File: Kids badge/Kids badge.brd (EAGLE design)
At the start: 3 parts

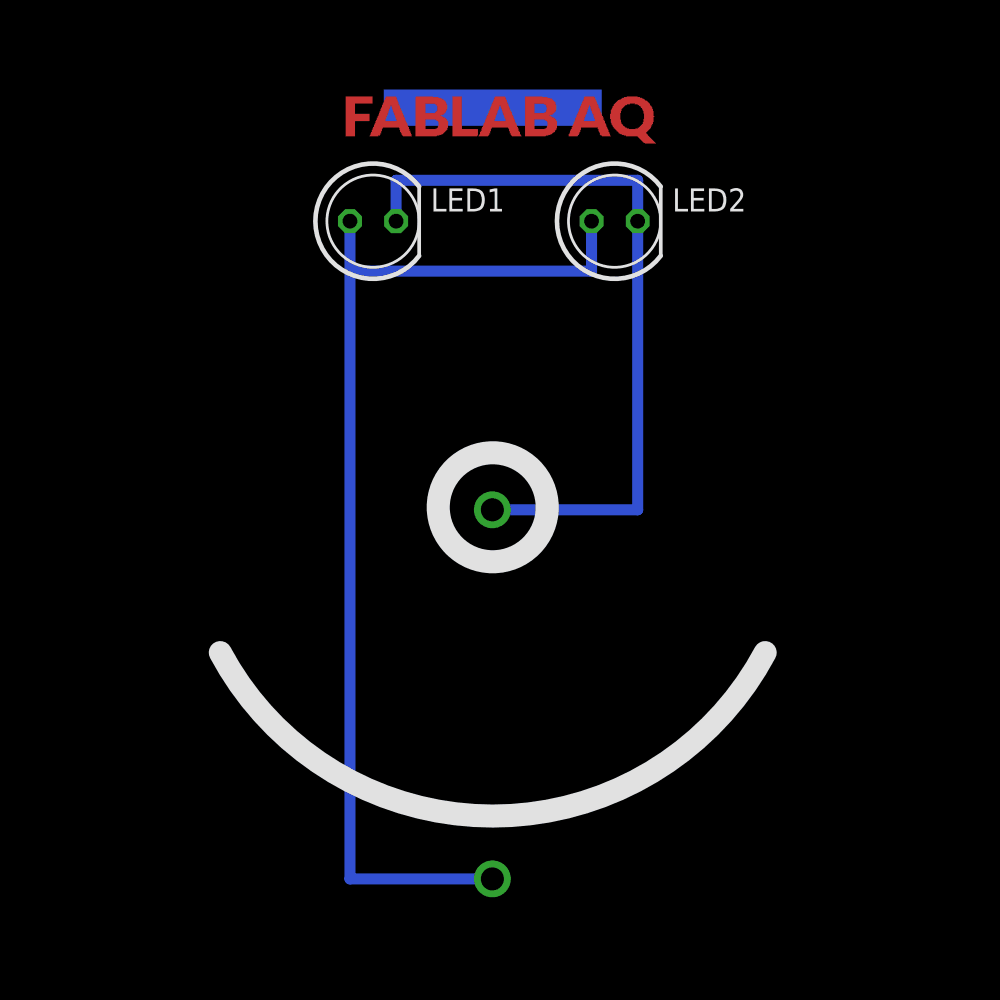
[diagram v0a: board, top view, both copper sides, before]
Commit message: new badges
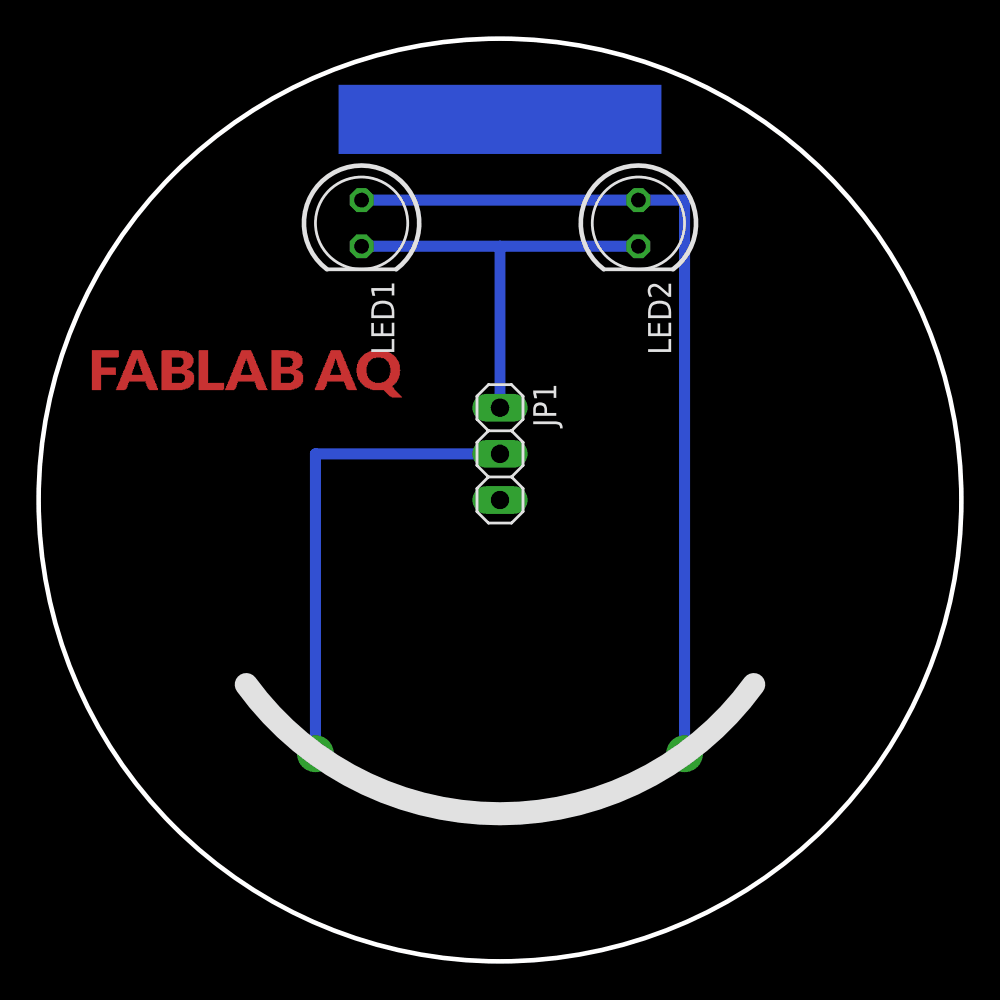
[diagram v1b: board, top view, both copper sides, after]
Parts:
- added JP1: (no value), pinhead:1X03
- BATT: value (none) -> BATTERY_1236_C
- moved BATT 12.6 mm to (35.6, 11.4), turned to 270 degrees
- moved LED2 1.31 mm to (33.0, 40.6), turned to 270 degrees
- moved LED1 0.64 mm to (17.8, 40.6), turned to 270 degrees
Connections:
- new net N$3: BATT.-, JP1.2
- net N$2: now also JP1.1; no longer BATT.-
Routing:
- net N$3: track 0.00 -> 26.7 mm
- net N$2: track 41.7 -> 24.1 mm
- net N$1: track 60.1 -> 48.3 mm
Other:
- board outline added: 50.8 x 50.8 mm

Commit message: routed PCBs
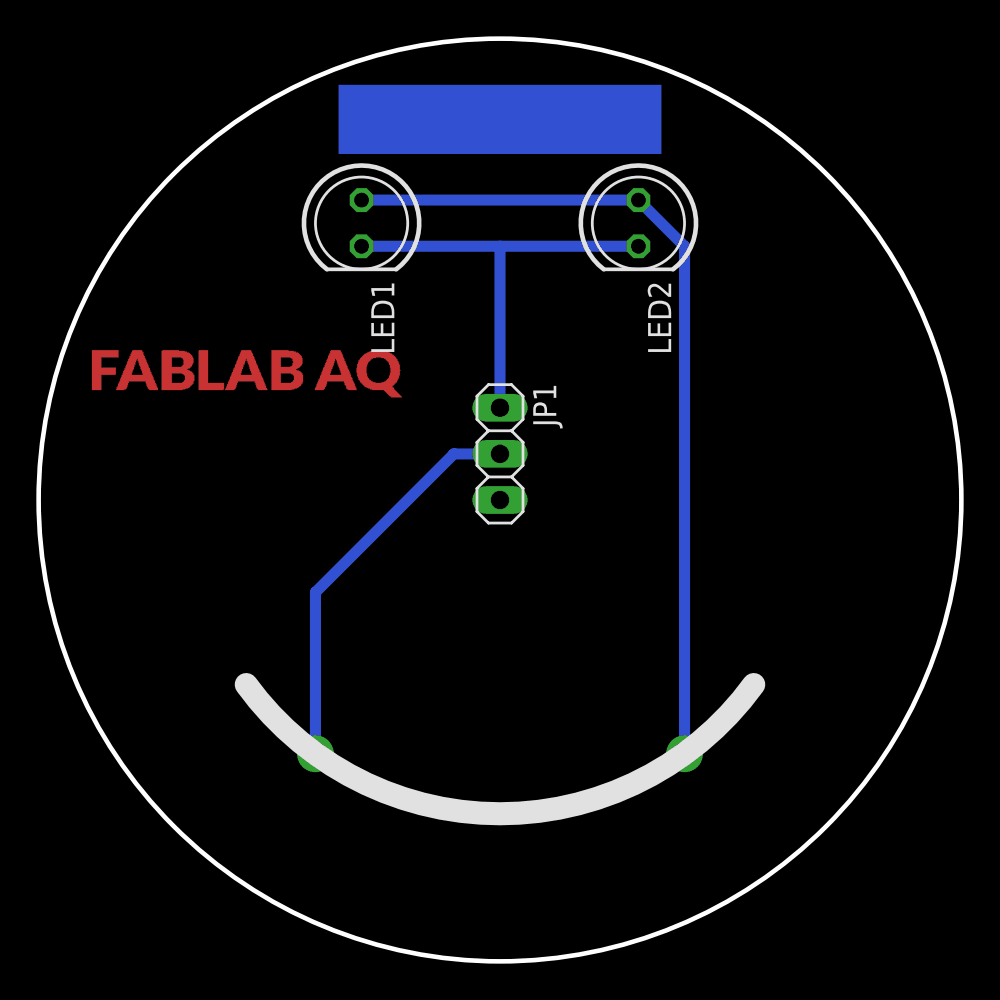
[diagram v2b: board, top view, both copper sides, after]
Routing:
- net N$3: track 26.7 -> 22.2 mm
- net N$1: track 48.3 -> 46.8 mm
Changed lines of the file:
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@@
 <contactref element="LED1" pad="A"/>
 <contactref element="BATT" pad="+"/>
-<wire x1="35.56" y1="11.43" x2="35.56" y2="41.91" width="0.6096" layer="16"/>
-<wire x1="35.56" y1="41.91" x2="33.02" y2="41.91" width="0.6096" layer="16"/>
 <wire x1="33.02" y1="41.91" x2="17.78" y2="41.91" width="0.6096" layer="16"/>
+<wire x1="33.02" y1="41.91" x2="35.56" y2="39.37" width="0.6096" layer="16"/>
+<wire x1="35.56" y1="39.37" x2="35.56" y2="11.43" width="0.6096" layer="16"/>
 </signal>
 <signal name="N$2">
@@
 <contactref element="BATT" pad="-"/>
 <contactref element="JP1" pad="2"/>
-<wire x1="15.24" y1="11.43" x2="15.24" y2="27.94" width="0.6096" layer="16"/>
-<wire x1="15.24" y1="27.94" x2="25.4" y2="27.94" width="0.6096" layer="16"/>
+<wire x1="15.24" y1="11.43" x2="15.24" y2="20.32" width="0.6096" layer="16"/>
+<wire x1="15.24" y1="20.32" x2="22.86" y2="27.94" width="0.6096" layer="16"/>
+<wire x1="22.86" y1="27.94" x2="25.4" y2="27.94" width="0.6096" layer="16"/>
 </signal>
 </signals>
